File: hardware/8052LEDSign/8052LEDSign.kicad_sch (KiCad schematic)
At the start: 22 parts, among them J1 TTL Serial, SW1 SW_SPST, U1 MSM83C154, U2 74LS75, U3 74LS75, U4 CY62256-70PC, U5 74LS08, U6 74LS10, U7 ATmega328-P, Y1 13.875 MHz

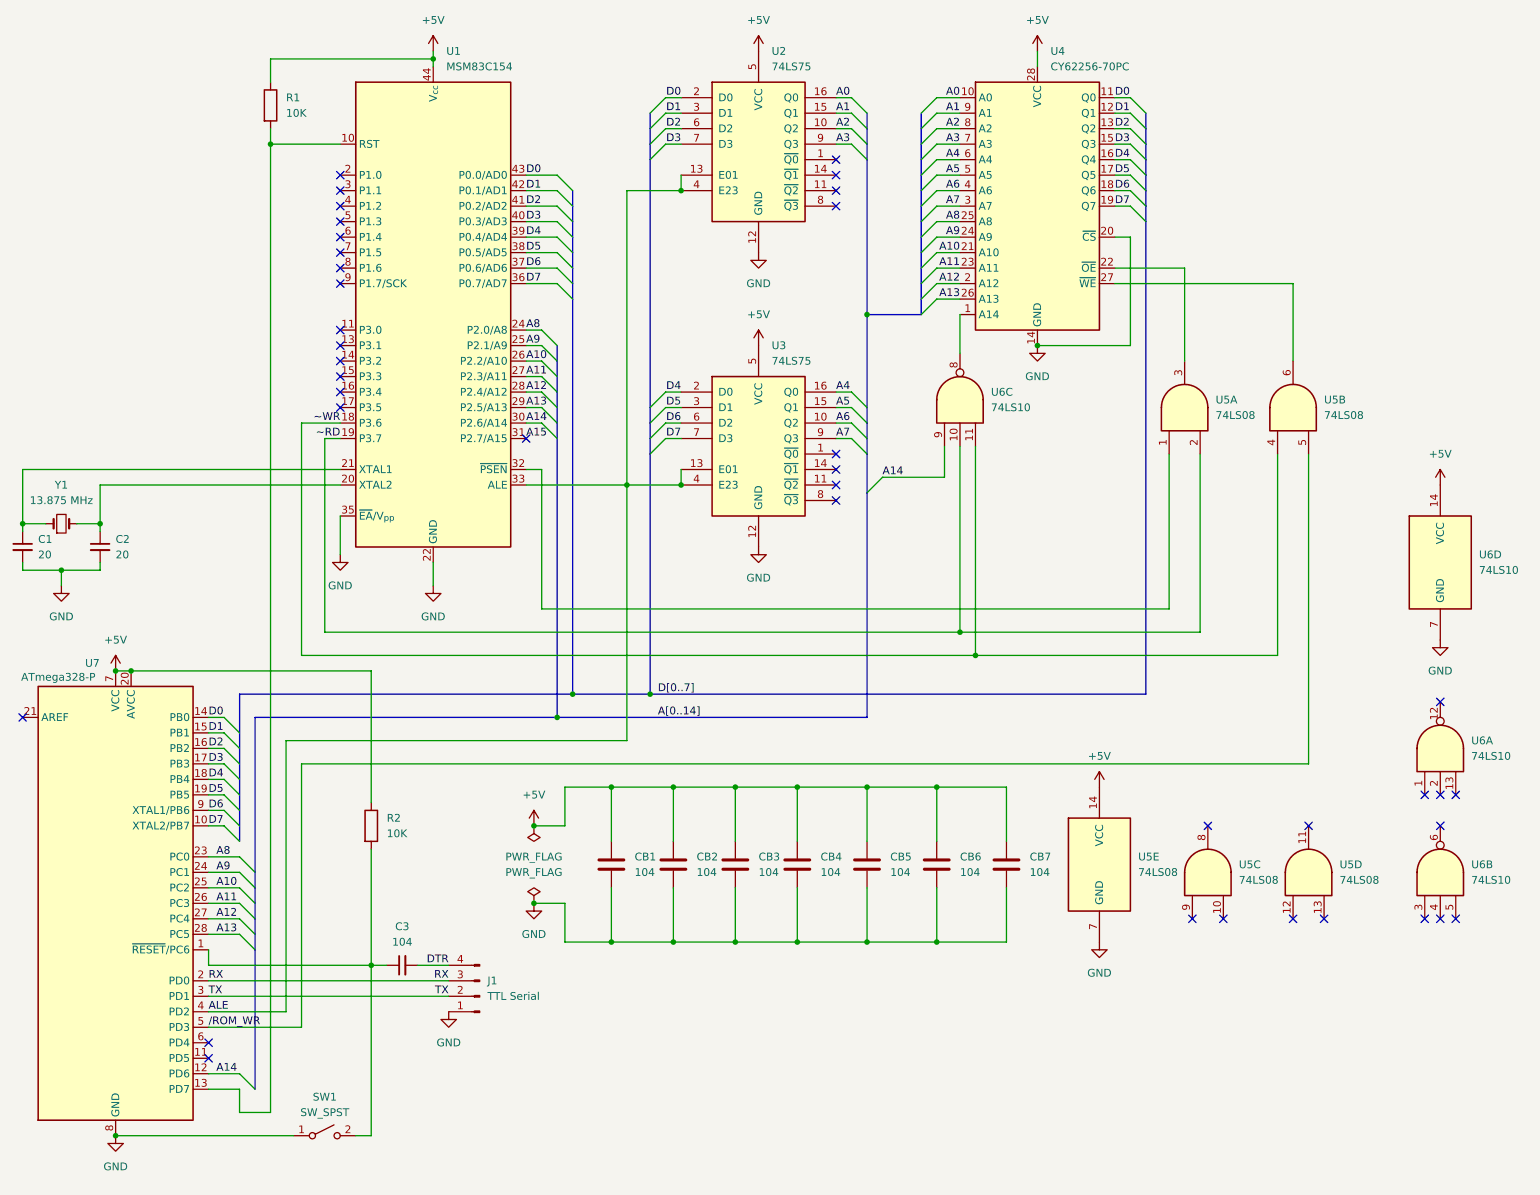
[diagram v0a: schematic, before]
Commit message: BLINKING IS WORKING!
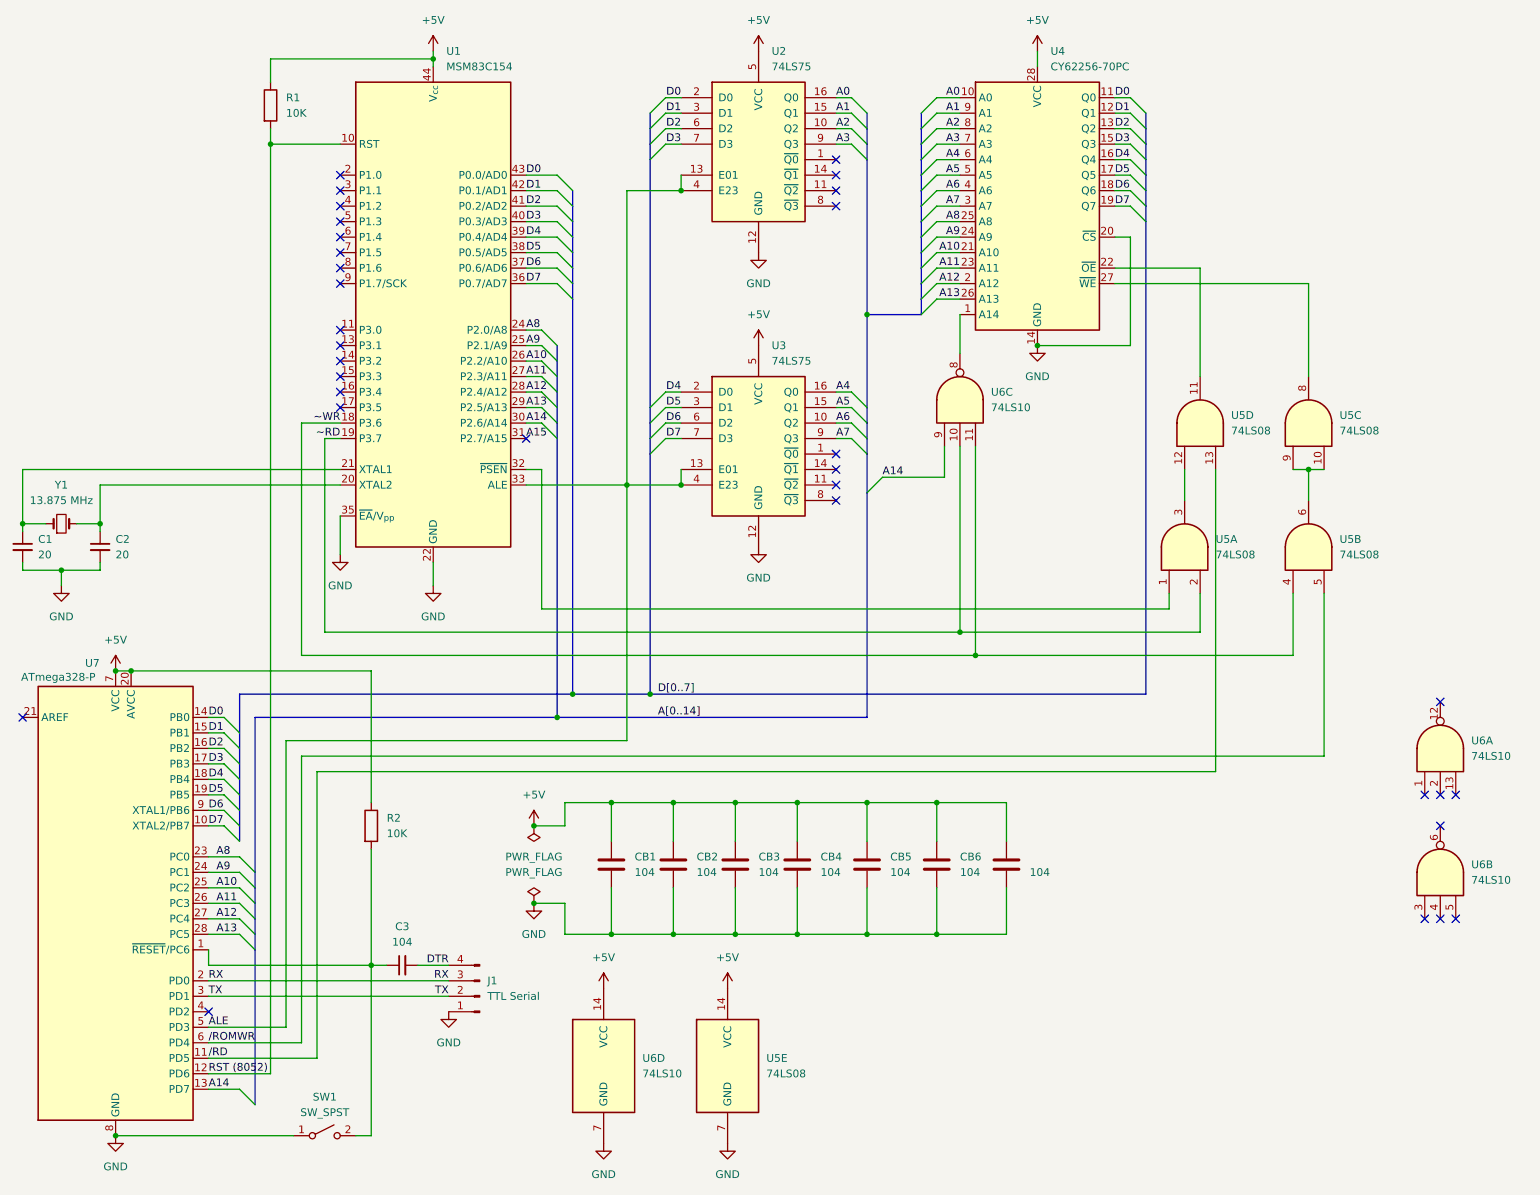
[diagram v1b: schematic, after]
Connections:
- net A14: now also U7.13 (PD7); no longer U7.12 (PD6)
- net ALE: now also U7.5 (PD3); no longer U7.4 (PD2)
- net at U5.10: now also U5.6, U5.9
- net at U5.8: now also U4.27 (~{WE})
- net RST (8052): now reaches R1.2, U1.10 (RST)
- net RST (8052): now also U7.12 (PD6); no longer U7.13 (PD7)
- net at U5.3: now also U5.12; no longer U4.22 (~{OE})
- net at U5.11: now also U4.22 (~{OE})
- net /RD: now reaches U5.13
- net /RD: now also U7.11 (PD5)
- net /ROMWR: now reaches U7.6 (PD4)
- net /ROMWR: now also U5.5
- removed net /ROM_WR: U5.5, U7.5 (PD3)
- no-connect marks 40 -> 33
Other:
- moved on the sheet: U5A, U5B, U5C, U5D, U5E, U6D
